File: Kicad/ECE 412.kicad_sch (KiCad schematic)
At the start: 46 parts, among them IC1 ADG412, J1 Faraday Cup IN, U1 LM7805_TO220, U4 LMC662, U5 MAX1032BEUG_

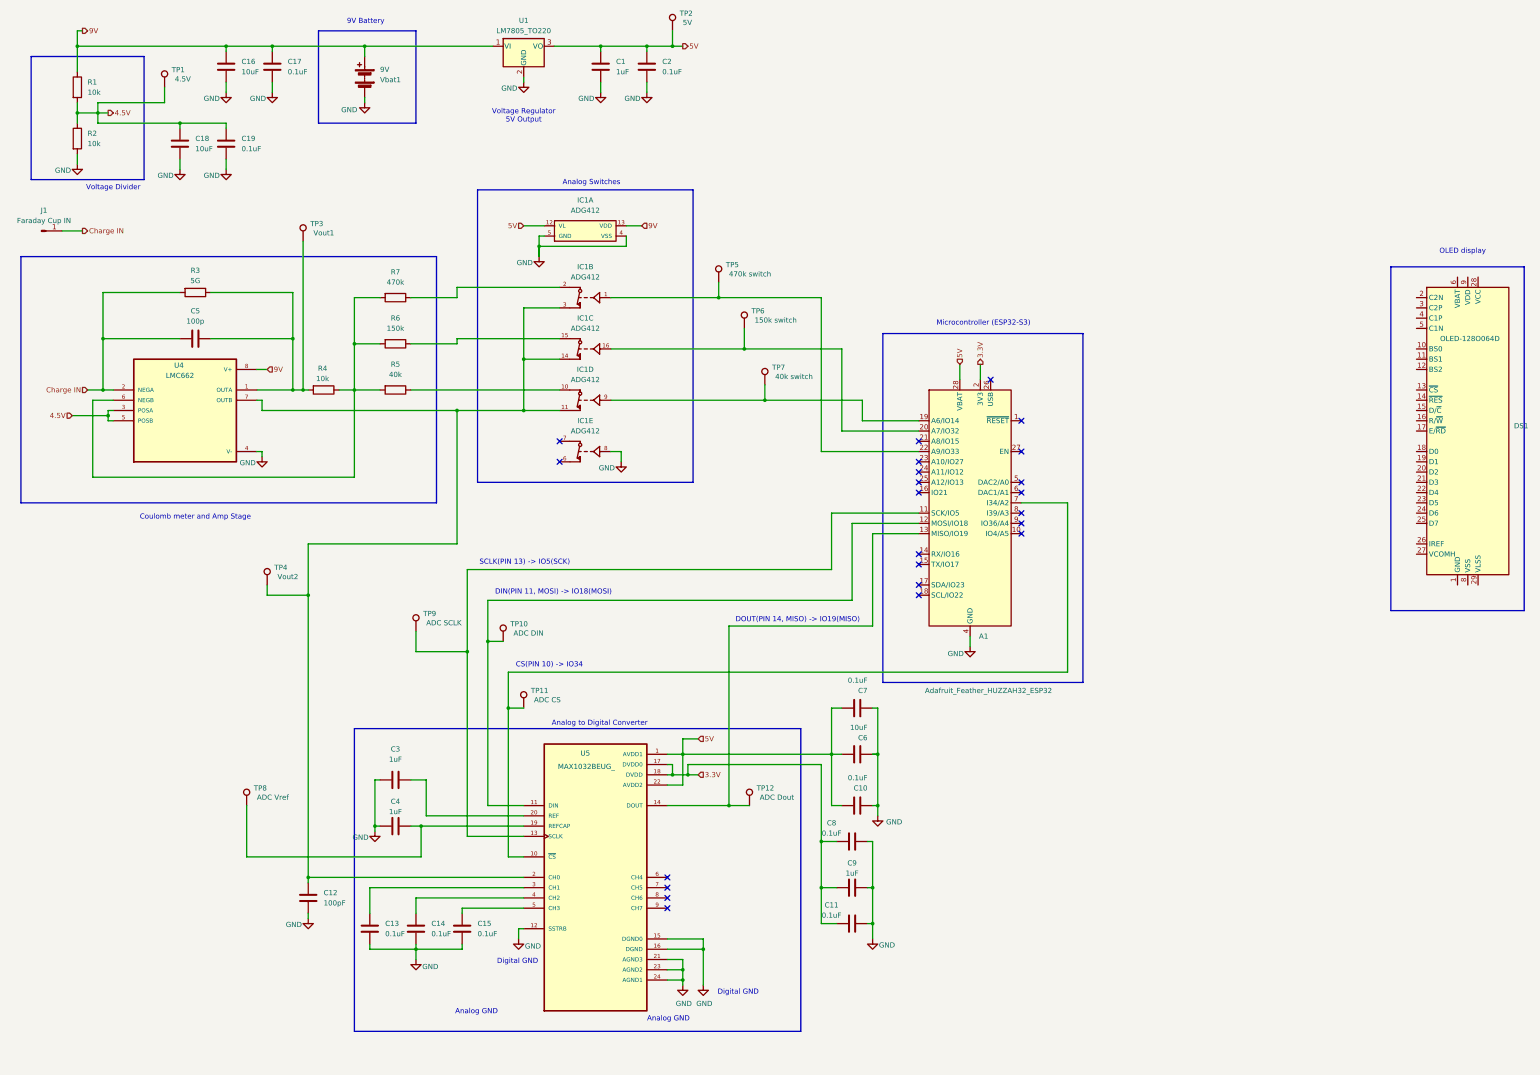
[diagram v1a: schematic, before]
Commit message: Add files via upload
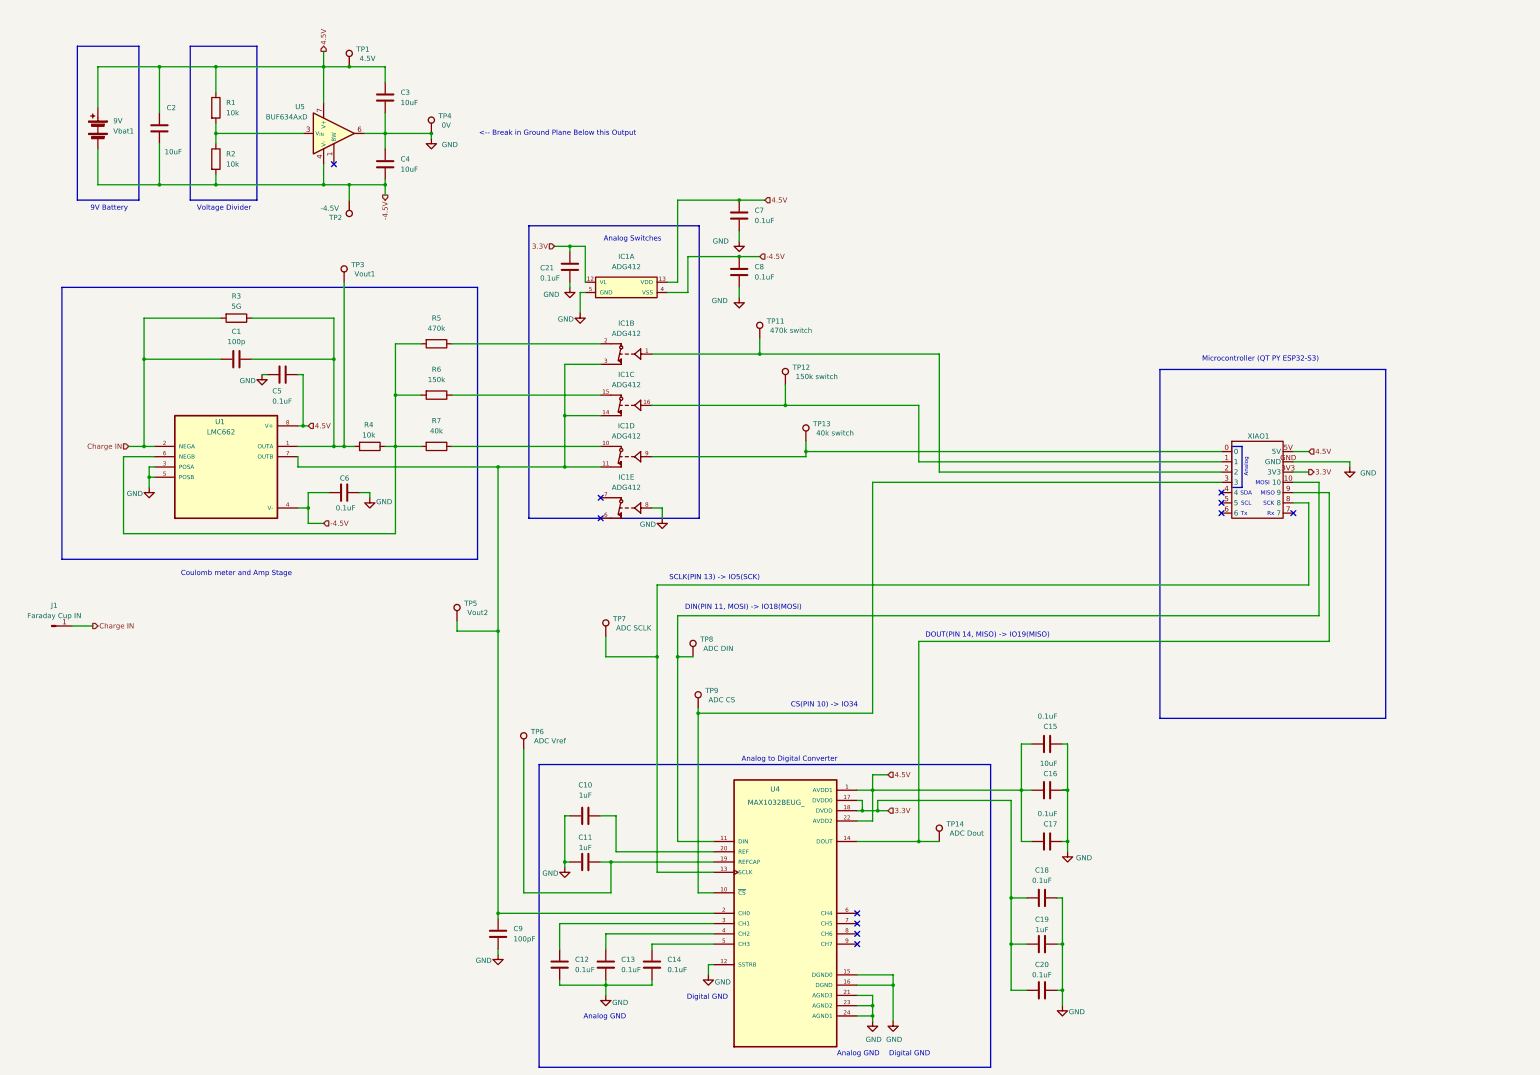
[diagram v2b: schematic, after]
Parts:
- removed A1: Adafruit_Feather_HUZZAH32_ESP32, Module:Adafruit_Feather, symbol MCU_Module:Adafruit_Feather_HUZZAH32_ESP32
- removed DS1: OLED-128O064D, Display:OLED-128O064D, symbol Display_Graphic:OLED-128O064D
- removed TP10: ADC DIN, TestPoint:TestPoint_THTPad_D2.0mm_Drill1.0mm, symbol Connector:TestPoint
- removed U1: LM7805_TO220, Package_TO_SOT_THT:TO-220-3_Vertical, symbol Regulator_Linear:LM7805_TO220
- removed U4: LMC662, Package_DIP:DIP-8_W7.62mm, symbol LMC6042IM:LMC6042IM
- removed U5: MAX1032BEUG_, MAX1032BEUGT:SOP65P640X110-24N, symbol MAX1032BEUG_:MAX1032BEUG_
- added C20, C21: 0.1uF, Capacitor_SMD:C_1206_3216Metric_Pad1.33x1.80mm_HandSolder, symbol Device:C
- added TP13: 40k switch, TestPoint:TestPoint_THTPad_D2.0mm_Drill1.0mm, symbol Connector:TestPoint
- added TP14: ADC Dout, TestPoint:TestPoint_THTPad_D2.0mm_Drill1.0mm, symbol Connector:TestPoint
- added U1: LMC662, Package_DIP:DIP-8_W7.62mm, symbol LMC6042IM:LMC6042IM
- added U4: MAX1032BEUG_, MAX1032BEUGT:SOP65P640X110-24N, symbol MAX1032BEUG_:MAX1032BEUG_
- added U5: BUF634AxD, Package_SO:SOIC-8_3.9x4.9mm_P1.27mm, symbol buf634axd:BUF634AxD
- added XIAO1: ~, XIAO_:XIAO_QTpy, symbol XIAO:esp32s3
- C1: value 1uF -> 100p; footprint Capacitor_SMD:C_1206_3216Metric_Pad1.33x1.80mm_HandSolder -> Capacitor_THT:C_Radial_D10.0mm_H12.5mm_P5.00mm
- C10, C11, C19: value 0.1uF -> 1uF
- C12: value 100pF -> 0.1uF
- C18, C6: value 10uF -> 0.1uF
- C2: value 0.1uF -> 10uF
- C3, C4: value 1uF -> 10uF
- C5: value 100p -> 0.1uF; footprint Capacitor_THT:C_Radial_D10.0mm_H12.5mm_P5.00mm -> Capacitor_SMD:C_1206_3216Metric_Pad1.33x1.80mm_HandSolder
- C9: value 1uF -> 100pF
- R5: value 40k -> 470k
- R7: value 470k -> 40k
- TP11: value ADC CS -> 470k switch
- TP12: value ADC Dout -> 150k switch
- TP2: value 5V -> -4.5V
- TP4: value Vout2 -> 0V
- TP5: value 470k switch -> Vout2
- TP6: value 150k switch -> ADC Vref
- TP7: value 40k switch -> ADC SCLK
- TP8: value ADC Vref -> ADC DIN
- TP9: value ADC SCLK -> ADC CS
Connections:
- net 9V is gone; now on net 4.5V: C16.1, C17.1, IC1.13 (VDD), R1.1, Vbat1.1 (+)
- net 3.3V: now also C18.2, C19.1, IC1.12 (VL), C20.2, C21.1, U4.17 (DVDD0), U4.18 (DVDD), XIAO1.3V3; no longer C11.2, C8.2, C9.1
- net 4.5V: now also C15.1, C2.1, C3.1, C5.1, C7.1, U1.8 (V+), U4.1 (AVDD1), U4.22 (AVDD2), U5.7 (V+), XIAO1.5V; no longer C18.1, C19.1, R1.2, R2.1
- net Charge IN: now also C1.2, U1.2 (NEGA); no longer C5.2
- net GND: now also C10.1, C11.2, C15.2, C18.1, C3.2, C4.1, C5.2, C8.2, C9.1, TP4.1, C20.1, C21.2, U1.3 (POSA), U1.5 (POSB), U4.12 (SSTRB), U4.15 (DGND0), U4.16 (DGND), U4.21 (AGND3), U4.23 (AGND2), U4.24 (AGND1), U5.6, XIAO1.GND; no longer C1.2, C10.2, C11.1, C15.1, C18.2, C2.2, C3.1, C4.2, C8.1, C9.2, IC1.4 (VSS), R2.2, Vbat1.2 (-)
- net at TP7.1: now also U4.13 (SCLK), XIAO1.8; no longer IC1.9
- net at IC1.11, IC1.14, IC1.3: now also C9.2, TP5.1, U1.7 (OUTB), U4.2 (CH0); no longer C12.2, TP4.1
- net at IC1.10: now also R7.1; no longer R5.1
- net at IC1.2: now also R5.1; no longer R7.1
- net at R4.1, R5.2, R6.2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: now also U1.6 (NEGB)
- net at R3.1, R4.2, TP3.1: now also C1.1, U1.1 (OUTA); no longer C5.1
- net at IC1.1: now also TP11.1, XIAO1.2; no longer TP5.1
- net at C14.2: now also U4.5 (CH3)
- net at TP12.1: now also IC1.16, XIAO1.1
- net at TP6.1: now also C11.1, U4.19 (REFCAP); no longer IC1.16
- net at TP8.1: now also U4.11 (DIN), XIAO1.10; no longer C4.1
- net at TP9.1: now also U4.10 (~{CS}), XIAO1.3
- net at C13.2: now also U4.4 (CH2)
- removed net 5V: C1.1, C10.1, C2.1, C6.1, C7.1, IC1.12 (VL), TP2.1
- new net: R1.2, R2.1, U5.3 (V_{IN})
- new net: C12.2, U4.3 (CH1)
- new net: TP14.1, U4.14 (DOUT), XIAO1.9
- new net: C10.2, U4.20 (REF)
- new net: IC1.9, TP13.1, XIAO1.0
- new net -4.5V: C2.2, C4.2, C6.1, C8.1, IC1.4 (VSS), R2.2, TP2.1, U1.4 (V-), U5.4 (V-), Vbat1.2 (-)
- no-connect marks 23 -> 11
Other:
- note added: "<-- Break in Ground Plane Below this Output"
- note added: "Analog"
- note added: "MISO"
- note added: "MOSI"
- note added: "Microcontroller (QT PY ESP32-S3)"
- note added: "Rx"
- note added: "SCK"
- note added: "SCL"
- note added: "SDA"
- note added: "Tx"
- note removed: "Microcontroller (ESP32-S3)"
- note removed: "OLED display"
- note removed: "Voltage Regulator 5V Output"
